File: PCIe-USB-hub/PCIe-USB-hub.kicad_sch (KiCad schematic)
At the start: 137 parts, among them J1 USB3_A, J10 USB3_A, J11 USB3_A, J12 Barrel_Jack_MountingPin, J2 USB3_A, J3 USB3_A, J4 USB3_A, J5 PCIexpress_x1, J6 USB3_A, J7 USB3_A, J8 USB3_A, J9 USB3_A

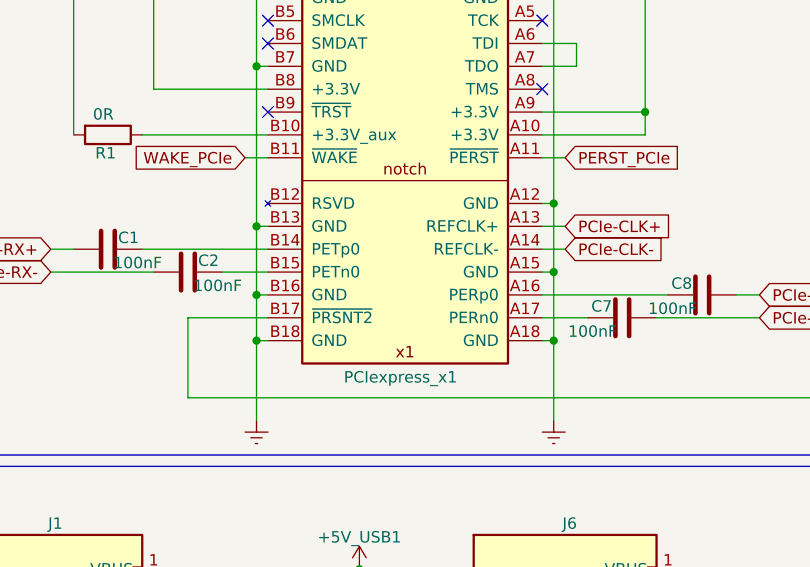
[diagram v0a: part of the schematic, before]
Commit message: натыкал трассировку всех дифф линий, поменял часть местами для удобной трассировки
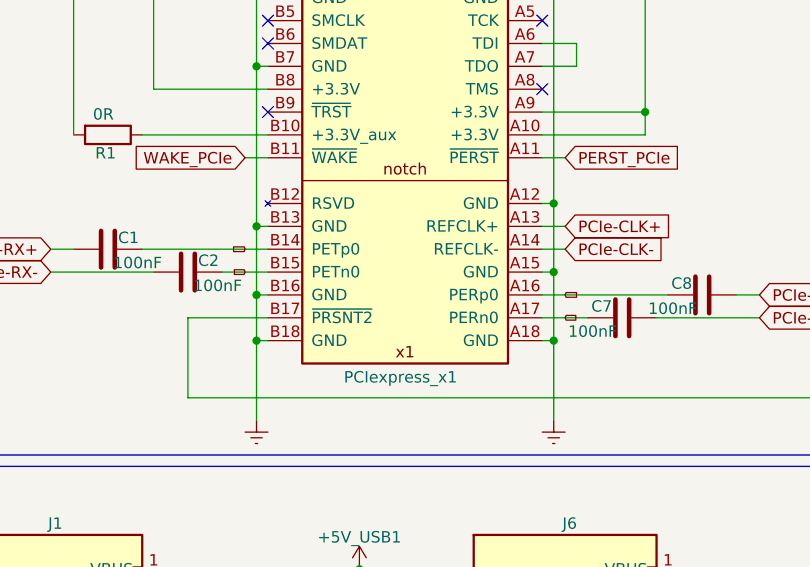
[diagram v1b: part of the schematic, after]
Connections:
- net _PCIe-RX-: now reaches C2.2, J5.B15 (PETn0)
- net _PCIe-TX-: now reaches C7.2, J5.A17 (PERn0)
- net _PCIe-TX+: now reaches C8.2, J5.A16 (PERp0)
- net _PCIe-RX+: now reaches C1.2, J5.B14 (PETp0)
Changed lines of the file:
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@@
+		)
+	)
+	(global_label "_PCIe-RX+"
+		(shape input)
+		(at 60.96 77.47 180)
+		(fields_autoplaced yes)
+		(effects
+			(font
+				(size 0.127 0.127)
+			)
+			(justify right)
+		)
+		(property "Intersheetrefs" "${INTERSHEET_REFS}"
+			(at 59.5785 77.47 0)
+			(effects
+				(font
+					(size 1.27 1.27)
+				)
+				(justify right)
+				(hide yes)
+			)
 		)
 	)
@@
 		)
 	)
+	(global_label "_PCIe-RX-"
+		(shape input)
+		(at 60.96 80.01 180)
+		(fields_autoplaced yes)
+		(effects
+			(font
+				(size 0.127 0.127)
+			)
+			(justify right)
+		)
+		(property "Intersheetrefs" "${INTERSHEET_REFS}"
+			(at 59.5785 80.01 0)
+			(effects
+				(font
+					(size 1.27 1.27)
+				)
+				(justify right)
+				(hide yes)
+			)
+		)
+	)
 	(global_label "USB-downstream9-RX-"
 		(shape input)
@@
 		)
 	)
+	(global_label "_PCIe-TX+"
+		(shape input)
+		(at 96.52 82.55 0)
+		(fields_autoplaced yes)
+		(effects
+			(font
+				(size 0.127 0.127)
+			)
+			(justify left)
+		)
+		(property "Intersheetrefs" "${INTERSHEET_REFS}"
+			(at 97.8713 82.55 0)
+			(effects
+				(font
+					(size 1.27 1.27)
+				)
+				(justify left)
+				(hide yes)
+			)
+		)
+	)
 	(global_label "OCI6B"
 		(shape input)
@@
 		)
 	)
+	(global_label "_PCIe-TX-"
+		(shape input)
+		(at 96.52 85.09 0)
+		(fields_autoplaced yes)
+		(effects
+			(font
+				(size 0.127 0.127)
+			)
+			(justify left)
+		)
+		(property "Intersheetrefs" "${INTERSHEET_REFS}"
+			(at 97.8713 85.09 0)
+			(effects
+				(font
+					(size 1.27 1.27)
+				)
+				(justify left)
+				(hide yes)
+			)
+		)
+	)
 	(global_label "USB-downstream7-RX+"
 		(shape input)
@@
 				(justify left)
 				(hide yes)
+			)
+		)
+	)
+	(rule_area
+		(polyline
+			(pts
+				(xy 128.27 276.098) (xy 128.27 255.27) (xy 120.65 254) (xy 113.03 254) (xy 110.49 256.54) (xy 110.49 276.86)
+				(xy 113.03 279.4) (xy 120.65 279.4)
+			)
+			(stroke
+				(width 0)
+				(type dash)
+			)
+			(fill
+				(type none)
 			)
 		)
@@
 		(polyline
 			(pts
-				(xy 71.12 276.098) (xy 71.12 255.27) (xy 63.5 254) (xy 55.88 254) (xy 53.34 256.54) (xy 53.34 276.86)
-				(xy 55.88 279.4) (xy 63.5 279.4)
+				(xy 128.27 137.668) (xy 128.27 116.84) (xy 120.65 115.57) (xy 113.03 115.57) (xy 110.49 118.11)
+				(xy 110.49 138.43) (xy 113.03 140.97) (xy 120.65 140.97)
 			)
 			(stroke
@@
 		(polyline
 			(pts
-				(xy 191.77 137.668) (xy 191.77 116.84) (xy 184.15 115.57) (xy 176.53 115.57) (xy 173.99 118.11)
-				(xy 173.99 138.43) (xy 176.53 140.97) (xy 184.15 140.97)
+				(xy 71.12 276.098) (xy 71.12 255.27) (xy 63.5 254) (xy 55.88 254) (xy 53.34 256.54) (xy 53.34 276.86)
+				(xy 55.88 279.4) (xy 63.5 279.4)
+			)
+			(stroke
+				(width 0)
+				(type dash)
+			)
+			(fill
+				(type none)
+			)
+		)
+	)
+	(rule_area
+		(polyline
+			(pts
+				(xy 128.27 179.578) (xy 128.27 158.75) (xy 120.65 157.48) (xy 113.03 157.48) (xy 110.49 160.02)
+				(xy 110.49 180.34) (xy 113.03 182.88) (xy 120.65 182.88)
 			)
 			(stroke
@@
 		(polyline
 			(pts
-				(xy 128.27 137.668) (xy 128.27 116.84) (xy 120.65 115.57) (xy 113.03 115.57) (xy 110.49 118.11)
-				(xy 110.49 138.43) (xy 113.03 140.97) (xy 120.65 140.97)
-			)
-			(stroke
-				(width 0)
-				(type dash)
-			)
-			(fill
-				(type none)
-			)
-		)
-	)
-	(rule_area
-		(polyline
-			(pts
-				(xy 128.27 179.578) (xy 128.27 158.75) (xy 120.65 157.48) (xy 113.03 157.48) (xy 110.49 160.02)
-				(xy 110.49 180.34) (xy 113.03 182.88) (xy 120.65 182.88)
+				(xy 71.12 179.578) (xy 71.12 158.75) (xy 63.5 157.48) (xy 55.88 157.48) (xy 53.34 160.02) (xy 53.34 180.34)
+				(xy 55.88 182.88) (xy 63.5 182.88)
 			)
 			(stroke
@@
 		(polyline
 			(pts
-				(xy 71.12 179.578) (xy 71.12 158.75) (xy 63.5 157.48) (xy 55.88 157.48) (xy 53.34 160.02) (xy 53.34 180.34)
-				(xy 55.88 182.88) (xy 63.5 182.88)
+				(xy 191.77 137.668) (xy 191.77 116.84) (xy 184.15 115.57) (xy 176.53 115.57) (xy 173.99 118.11)
+				(xy 173.99 138.43) (xy 176.53 140.97) (xy 184.15 140.97)
 			)
 			(stroke
-				(width 0)
-				(type dash)
-			)
-			(fill
-				(type none)
-			)
-		)
-	)
-	(rule_area
-		(polyline
-			(pts
-				(xy 128.27 276.098) (xy 128.27 255.27) (xy 120.65 254) (xy 113.03 254) (xy 110.49 256.54) (xy 110.49 276.86)
-				(xy 113.03 279.4) (xy 120.65 279.4)
-			)
-			(stroke

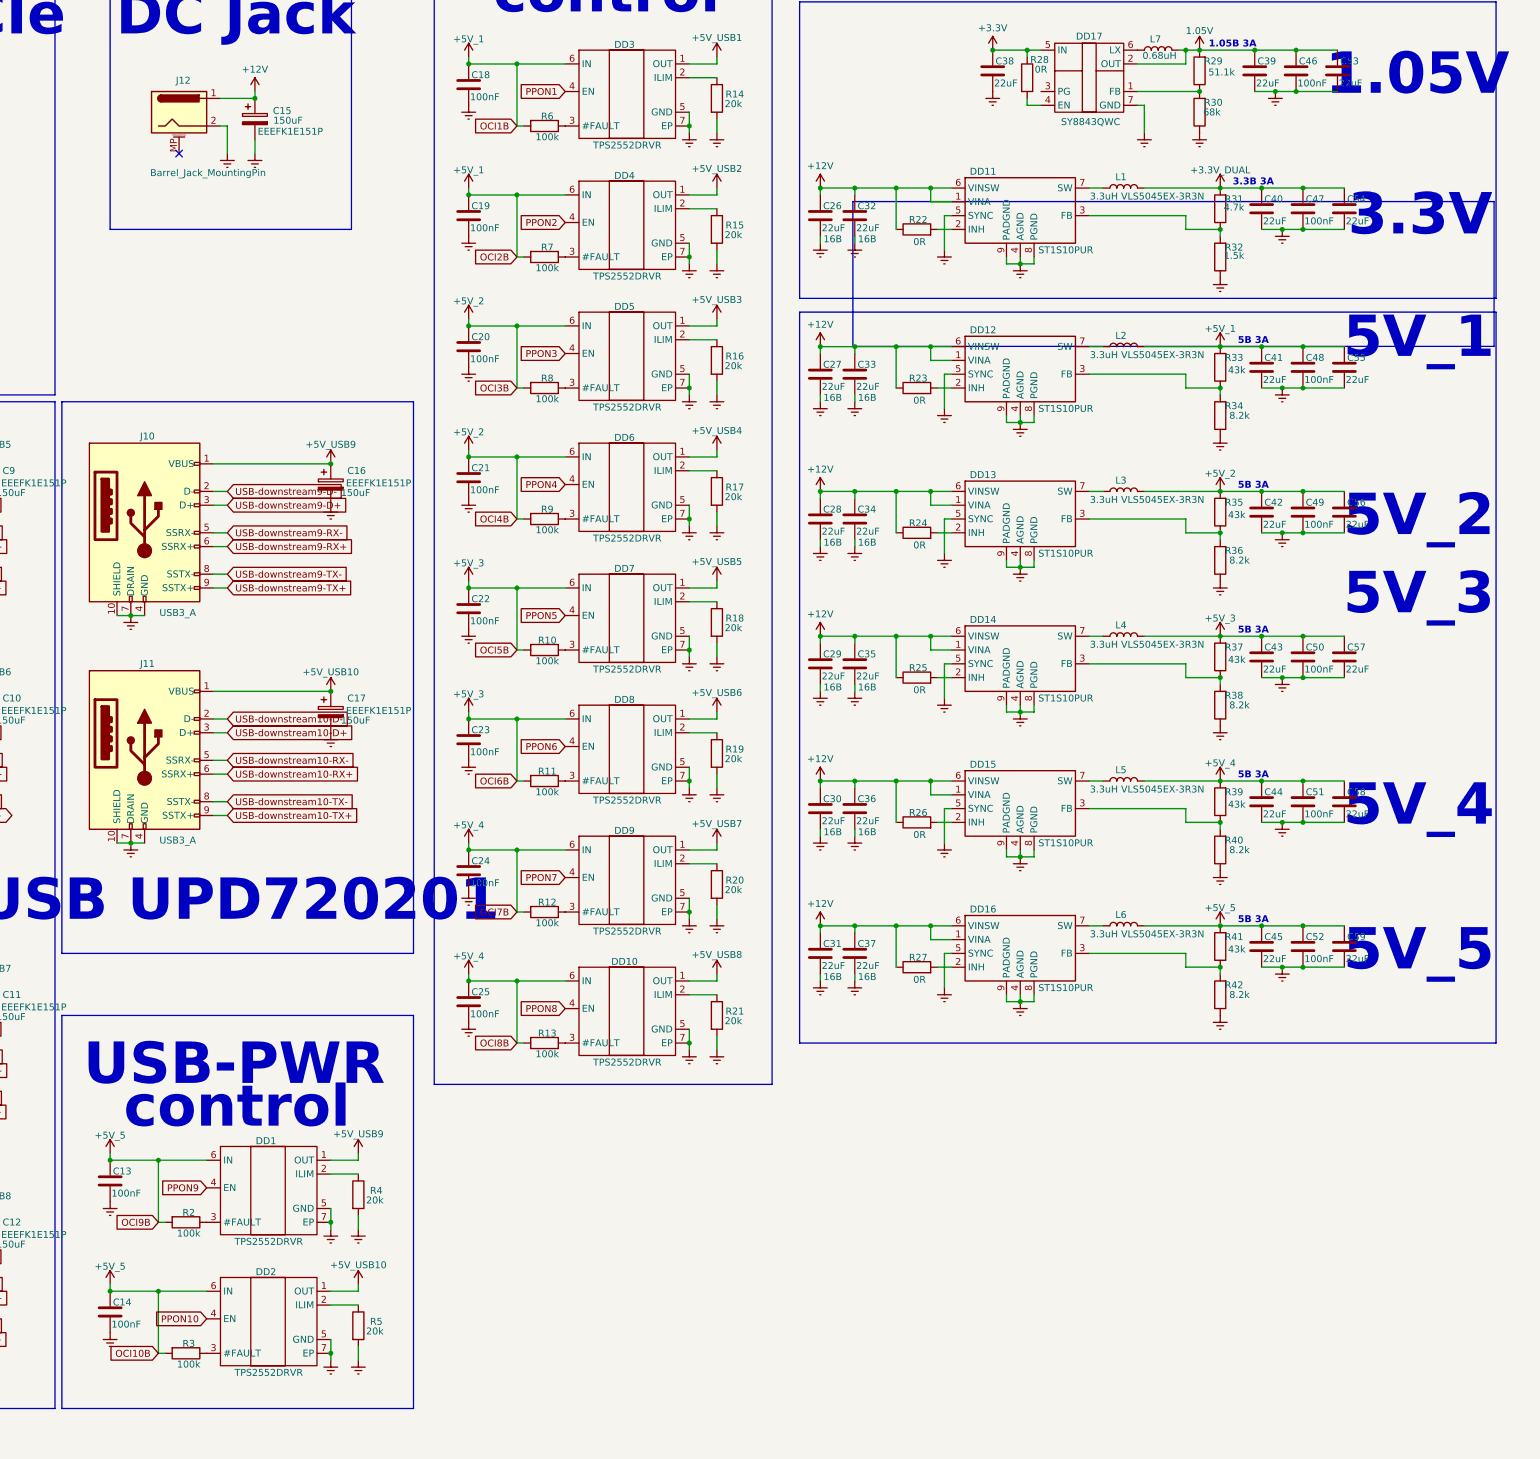
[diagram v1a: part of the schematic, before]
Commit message: тык-перетык
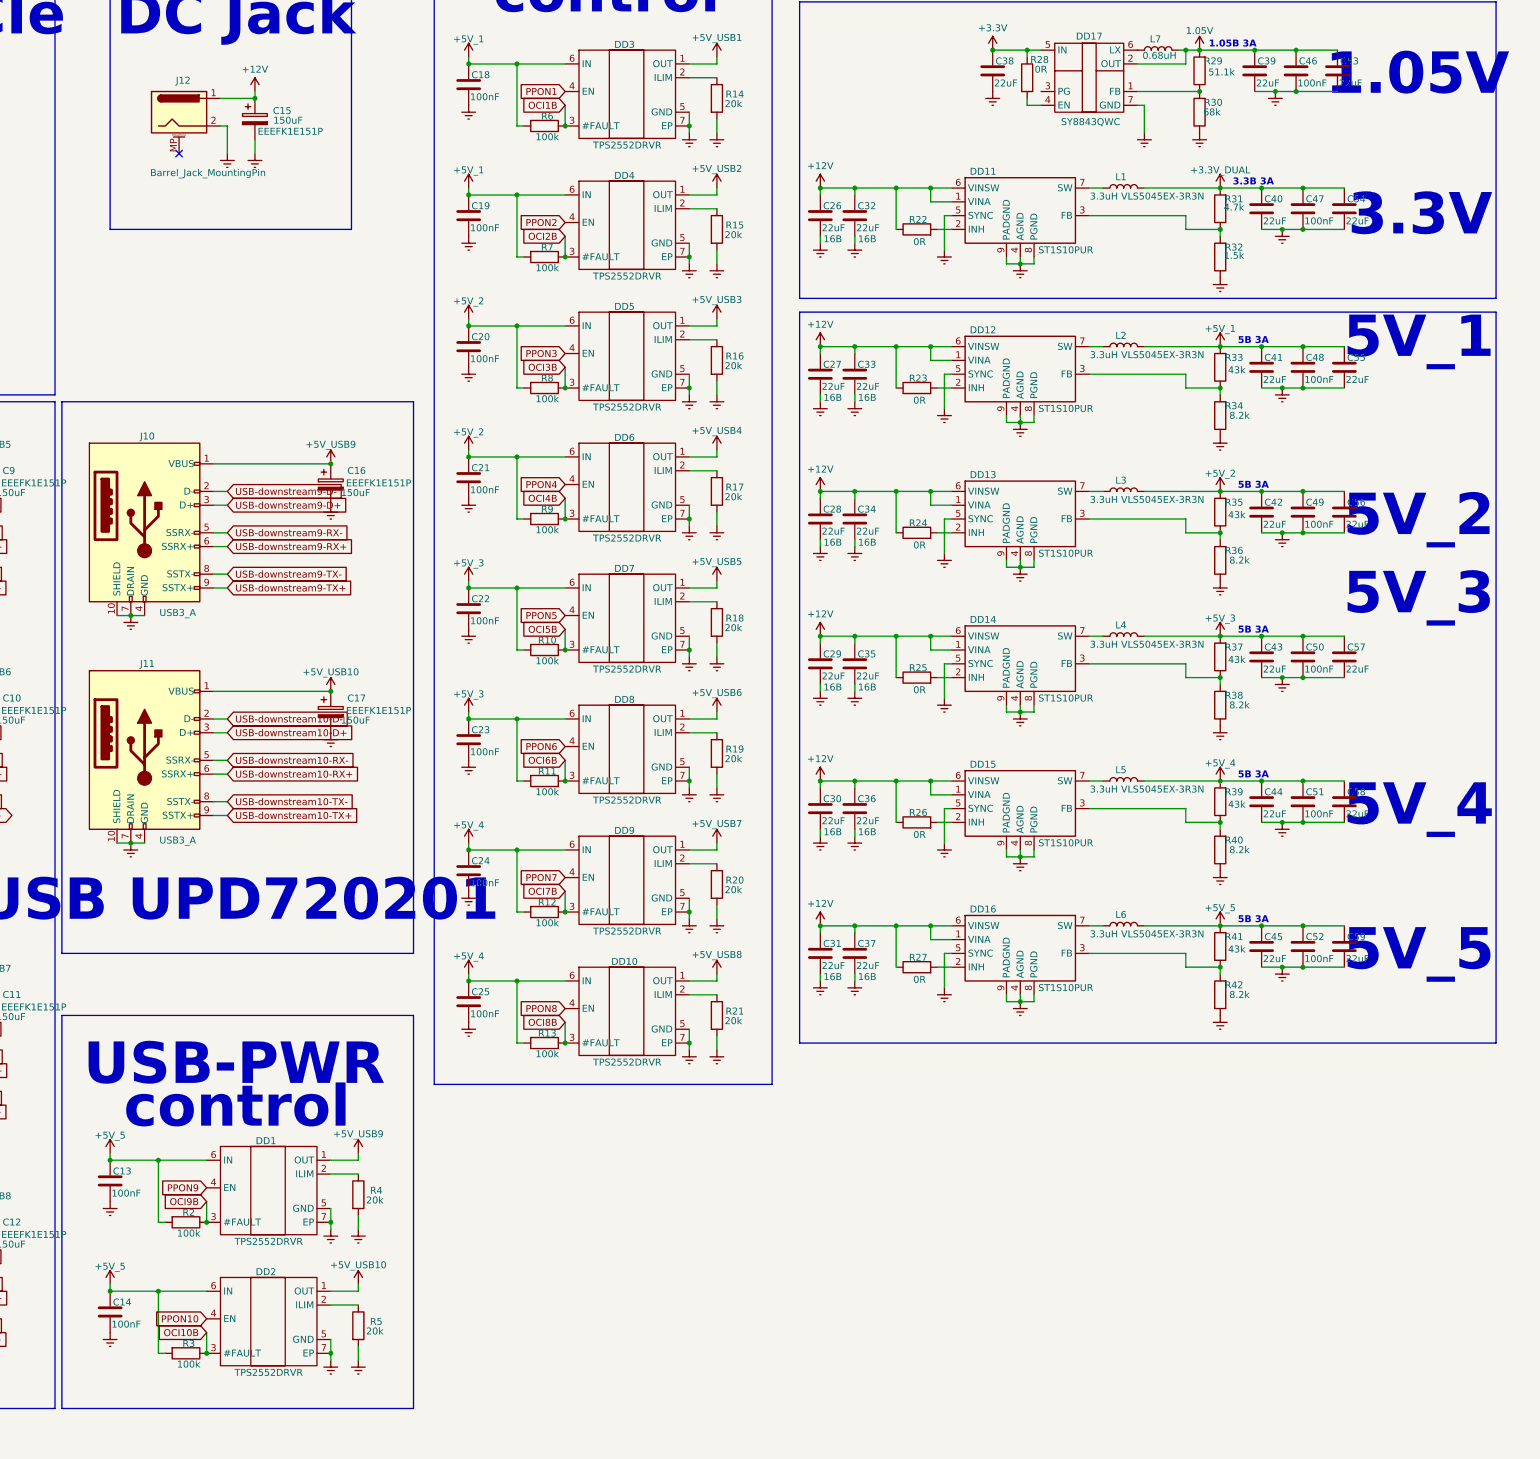
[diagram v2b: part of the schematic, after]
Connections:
- net OCI10B: now reaches DD2.3 (#FAULT), R3.1
- net OCI8B: now reaches DD10.3 (#FAULT), R13.1
- net OCI5B: now reaches DD7.3 (#FAULT), R10.1
- net OCI9B: now reaches DD1.3 (#FAULT), R2.1
- net OCI1B: now reaches DD3.3 (#FAULT), R6.1
- net OCI7B: now reaches DD9.3 (#FAULT), R12.1
- net OCI3B: now reaches DD5.3 (#FAULT), R8.1
- net OCI4B: now reaches DD6.3 (#FAULT), R9.1
- net OCI6B: now reaches DD8.3 (#FAULT), R11.1
- net OCI2B: now reaches DD4.3 (#FAULT), R7.1
